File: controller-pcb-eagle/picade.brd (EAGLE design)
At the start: 62.9 x 59 mm, 38 parts

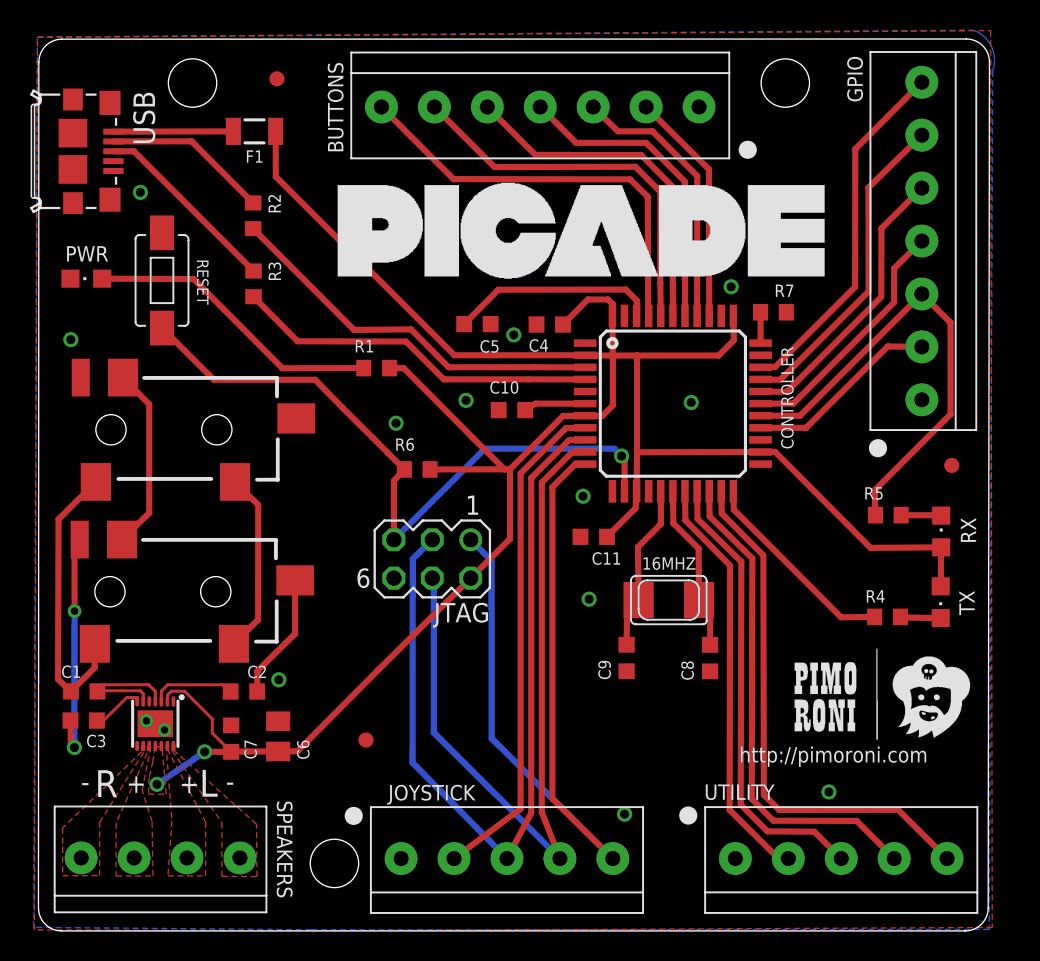
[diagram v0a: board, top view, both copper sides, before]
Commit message: Final Picade PCB layout
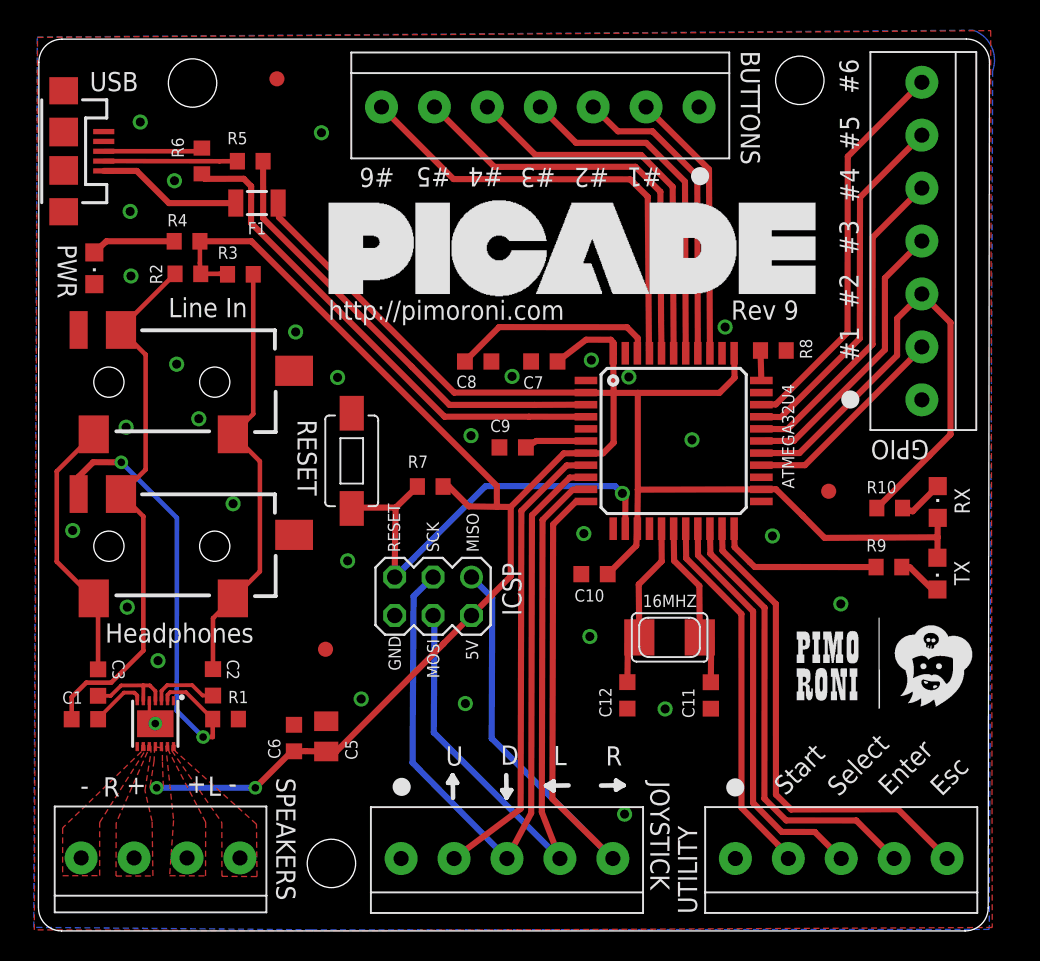
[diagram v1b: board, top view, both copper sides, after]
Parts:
- removed C4: 0.1µF, adafruit:C0603K
- removed CONTROLLER: ATMEGA32U4-AU, adafruit:TQFP44
- removed JTAG: (no value), con-lstb:MA03-2
- added ATMEGA32U4: ic-atmega32u4-tqfp44, adafruit:TQFP44
- added C12: cercap-22pF-0603, adafruit:C0603K
- added ICSP: (no value), con-lstb:MA03-2
- added R10, R9: res-1k-0603, resistor:R0603
- added R8: res-10k-0603, resistor:R0603
- 16MHZ: value (none) -> xtal-16mhz-5x3.2
- AMPLIFIER: value MAX98306ETD+ -> ic-max98306-tdfn14
- C1, C2, C3: value 1µF -> cercap-1uF-0603
- C10: value 1µF -> cercap-100nF-0603; device resistor:C0603K -> adafruit:C0603K
- C11: value 0.1µF -> cercap-22pF-0603
- C5: value 0.1µF -> cercap-10uF-0805; device adafruit:C0603K -> resistor:C0805K
- C6: value 10uF -> cercap-100nF-0603; device resistor:C0805K -> adafruit:C0603K
- C7: value 0.1µF -> cercap-100nF-0603
- C8: value 22pF -> cercap-100nf-0603
- C9: value 22pF -> cercap-1uF-0603; device adafruit:C0603K -> resistor:C0603K
- F1: value PTCSMD -> ptc-0.5A-120
- HEADPHONES: value AUDIO-JACK2SMD -> stereo-jack-switched; device SparkFun-Connectors:AUDIO-JACK-3.5MM-SMD -> pimoroni:AUDIO-JACK-3.5MM-SMD
- LINEIN: value (none) -> stereo-jack-noswitch
- PWR: value (none) -> led-white-0805
- R1: value 1kΩ -> res-470k-0603
- R2, R3: value 22Ω -> res-47k-0603
- R4: value 1kΩ -> res-1k-0603
- R5: value 1kΩ -> res-22-0603
- R6: value 10kΩ -> res-22-0603
- R7: value 10kΩ -> res-10k-0603
- RESET: value SWITCH-MOMENTARY-2-SMD-1101NE -> gullwing-switch
- RX: value (none) -> led-orange-0805
- TX: value (none) -> led-green-0805
- USB: value CON-USB-F-MICRO-B -> USB-REVERSE-MICROB; device dp_devices:CONN_USB_MICRO-B -> pimoroni:USB-MICROB
- moved R4 52.6 mm to (9.98, 45.9), turned to 0 degrees
- moved U$1 51.4 mm to (15.9, 56.6)
- moved R5 48.3 mm to (14.2, 51.2), turned to 0 degrees
- moved U$2 37.9 mm to (19.1, 18.9)
- moved U$3 34.7 mm to (52.4, 29.4)
- moved C7 32.4 mm to (33.6, 37.9), turned to 180 degrees
- moved C5 29.0 mm to (19.2, 13.2), turned to 90 degrees
- moved R7 25.5 mm to (26.1, 29.7), turned to 0 degrees
- moved R1 25.3 mm to (12.5, 14.3)
- moved C8 24.9 mm to (29.2, 37.9), turned to 180 degrees
- moved R6 24.9 mm to (11.0, 51.2), turned to 270 degrees
- moved RESET 17.3 mm to (20.9, 31.4)
- moved C9 15.8 mm to (31.5, 32.3), turned to 180 degrees
- moved C11 13.0 mm to (44.6, 15.9), turned to 90 degrees
- moved C10 12.1 mm to (36.9, 23.9)
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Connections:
- removed net N$43: HEADPHONES.TIP, LINEIN.TIP
- net GND: now also ATMEGA32U4.15, ATMEGA32U4.23, ATMEGA32U4.35, ATMEGA32U4.43, ATMEGA32U4.5, C11.1, C12.1, C5.2, C9.2, ICSP.6, R1.2, R8.1, USB.GND, USB.MT1, USB.MT2; no longer C11.2, C4.2, C5.1, C9.1, CONTROLLER.15, CONTROLLER.23, CONTROLLER.35, CONTROLLER.43, CONTROLLER.5, JTAG.6, R7.1, USB.P5
- net N$1: now also ATMEGA32U4.17, C11.2; no longer C8.2, CONTROLLER.17
- net N$10: now also ATMEGA32U4.22, R9.2; no longer CONTROLLER.22, R4.2
- net N$11: now also R9.1; no longer R4.1
- net N$12: now also R10.1; no longer R5.1
- net N$13: now also ATMEGA32U4.27, R10.2; no longer CONTROLLER.27, R5.2
- net N$14: now also ATMEGA32U4.11, ICSP.1; no longer CONTROLLER.11, JTAG.1
- net N$15: now also USB.VBUS; no longer USB.P1
- net N$16: now also ATMEGA32U4.9, ICSP.3; no longer CONTROLLER.9, JTAG.3
- net N$18: now also ATMEGA32U4.41; no longer CONTROLLER.41
- net N$19: now also ATMEGA32U4.40; no longer CONTROLLER.40
- net N$2: now also ATMEGA32U4.3, R5.2; no longer CONTROLLER.3, R2.2
- net N$20: now also ATMEGA32U4.39; no longer CONTROLLER.39
- net N$21: now also ATMEGA32U4.38; no longer CONTROLLER.38
- net N$22: now also ATMEGA32U4.37; no longer CONTROLLER.37
- net N$23: now also ATMEGA32U4.36; no longer CONTROLLER.36
- net N$24: now also ATMEGA32U4.21; no longer CONTROLLER.21
- net N$25: now also ATMEGA32U4.20; no longer CONTROLLER.20
- net N$26: now also ATMEGA32U4.19; no longer CONTROLLER.19
- net N$27: now also ATMEGA32U4.18; no longer CONTROLLER.18
- net N$28: now also ATMEGA32U4.8; no longer CONTROLLER.8
- net N$29: now also ATMEGA32U4.29; no longer CONTROLLER.29
- net N$3: now also R5.1, USB.D-; no longer R2.1, USB.P2
- net N$30: now also ATMEGA32U4.30; no longer CONTROLLER.30
- net N$31: now also ATMEGA32U4.31; no longer CONTROLLER.31
- net N$33: now also ATMEGA32U4.26; no longer CONTROLLER.26
- net N$34: now also ATMEGA32U4.28; no longer CONTROLLER.28
- net N$37: now also C1.1, HEADPHONES.RING, LINEIN.RING, R2.1; no longer C2.1, HEADPHONES.TSH
- net N$38: now also C2.1, HEADPHONES.TIP, LINEIN.TIP, R3.1; no longer C1.1, HEADPHONES.RSH
- net N$39: now also ATMEGA32U4.10, ICSP.4; no longer CONTROLLER.10, JTAG.4
- net N$4: now also R6.1, USB.D+; no longer R3.1, USB.P3
- net N$41: now also ATMEGA32U4.33, R8.2; no longer CONTROLLER.33, R7.2
- net N$42: now also AMPLIFIER.2, HEADPHONES.RSH, R1.1; no longer HEADPHONES.RING, LINEIN.RING
- net N$5: now also ATMEGA32U4.4, R6.2; no longer CONTROLLER.4, R3.2
- net N$6: now also ATMEGA32U4.6, C9.1; no longer C10.1, CONTROLLER.6
- net N$7: now also ATMEGA32U4.42, C8.2; no longer C5.2, CONTROLLER.42
- net N$8: now also ATMEGA32U4.16, C12.2; no longer C9.2, CONTROLLER.16
- net N$9: now also R4.1; no longer R1.1
- net RESET: now also ATMEGA32U4.13, ICSP.5, R7.1; no longer CONTROLLER.13, JTAG.5, R6.1
- net VCC: now also ATMEGA32U4.14, ATMEGA32U4.2, ATMEGA32U4.24, ATMEGA32U4.34, ATMEGA32U4.44, ATMEGA32U4.7, C10.1, C5.1, ICSP.2, R2.2, R3.2, R4.2, R7.2; no longer AMPLIFIER.2, C11.1, C4.1, CONTROLLER.14, CONTROLLER.2, CONTROLLER.24, CONTROLLER.34, CONTROLLER.44, CONTROLLER.7, JTAG.2, R1.2, R6.2
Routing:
- net N$37: track 8.39 -> 36.3 mm
- net N$42: track 12.2 -> 30.8 mm, vias 0 -> 2
- net RESET: track 45.0 -> 29.7 mm
- net N$9: track 19.7 -> 5.57 mm
- net N$38: track 15.7 -> 28.7 mm, vias 2 -> 0
- net N$43: track 12.0 -> 0.00 mm
- net VCC: track 154.8 -> 164.7 mm
- net N$5: track 24.2 -> 33.5 mm
- net N$4: track 12.5 -> 6.69 mm
- net N$14: track 54.0 -> 49.1 mm
- net N$39: track 50.8 -> 45.9 mm
- net N$16: track 54.4 -> 49.4 mm
- net N$2: track 25.8 -> 30.2 mm
- net N$26: track 30.1 -> 27.0 mm
- net N$25: track 32.6 -> 29.6 mm
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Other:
- board text added: "#1"
- board text added: "#2"
- board text added: "#3"
- board text added: "#4"
- board text added: "#5"
- board text added: "#6"
- board text added: "5V"
- board text added: "D"
- board text added: "Enter"
- board text added: "Esc"
- board text added: "GND"
- board text added: "Headphones"
- board text added: "Line In"
- board text added: "MISO"
- board text added: "MOSI"
- board text added: "RESET"
- board text added: "Rev 9"
- board text added: "SCK"
- board text added: "Select"
- board text added: "Start"
- board text added: "U"
